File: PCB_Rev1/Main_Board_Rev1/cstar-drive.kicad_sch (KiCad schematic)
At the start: 2 parts, among them J12 532610771, J9 532610771

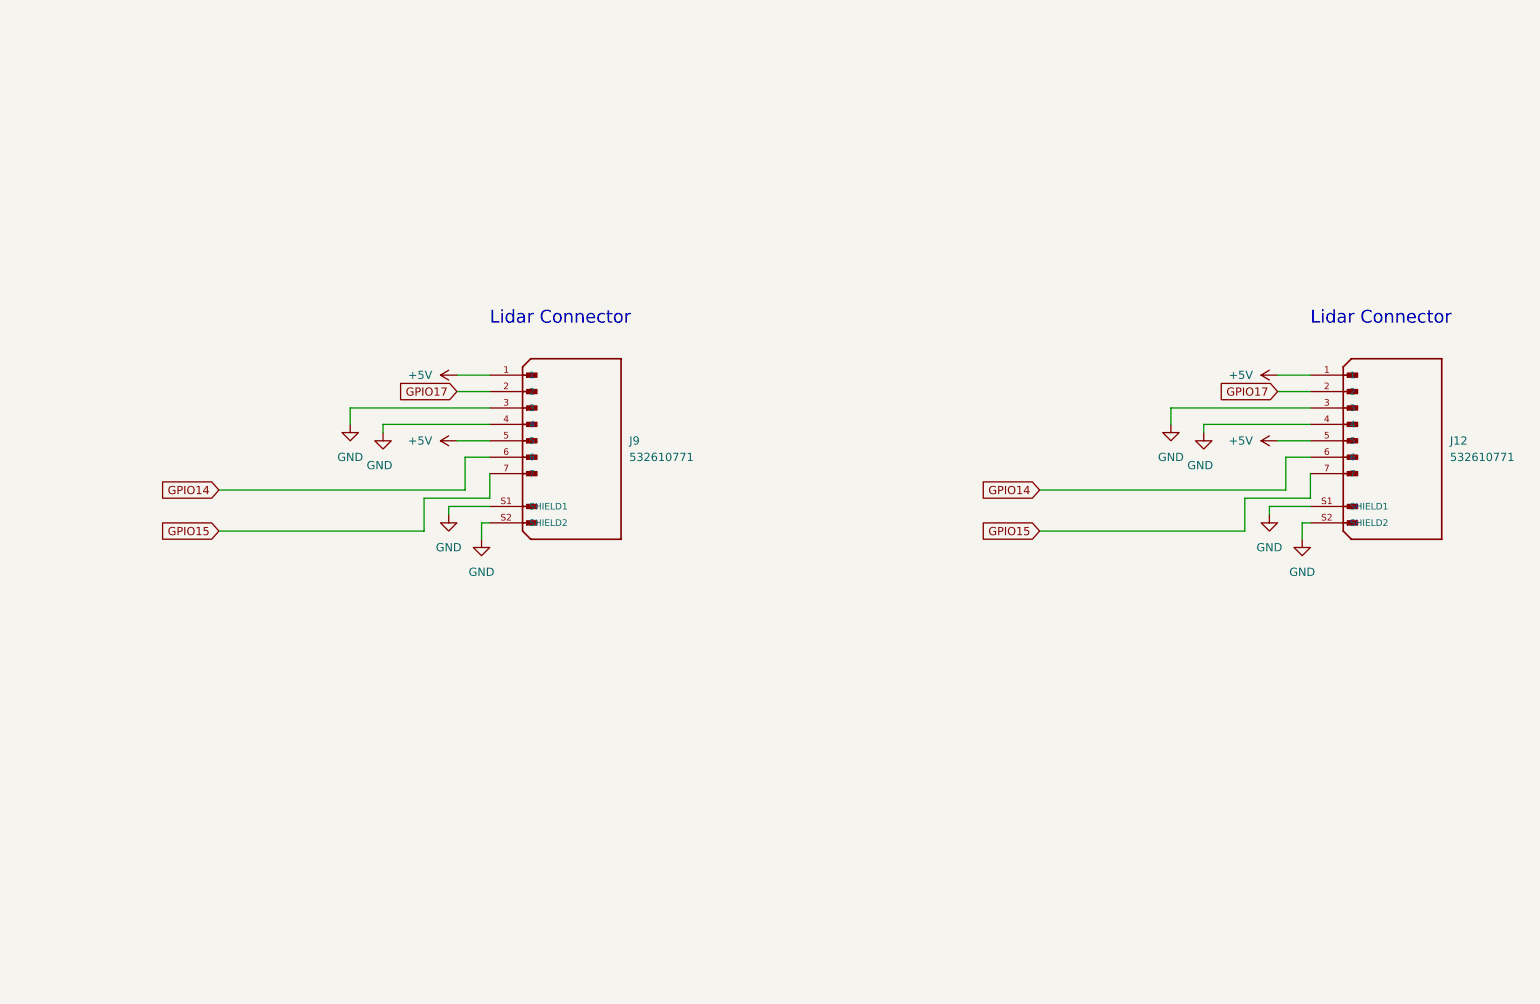
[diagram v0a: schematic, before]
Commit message: Revert "Audio subsystem re-created"
This reverts commit 6dc47edf88eae56b01440ce5f2dfd5da155ce597.
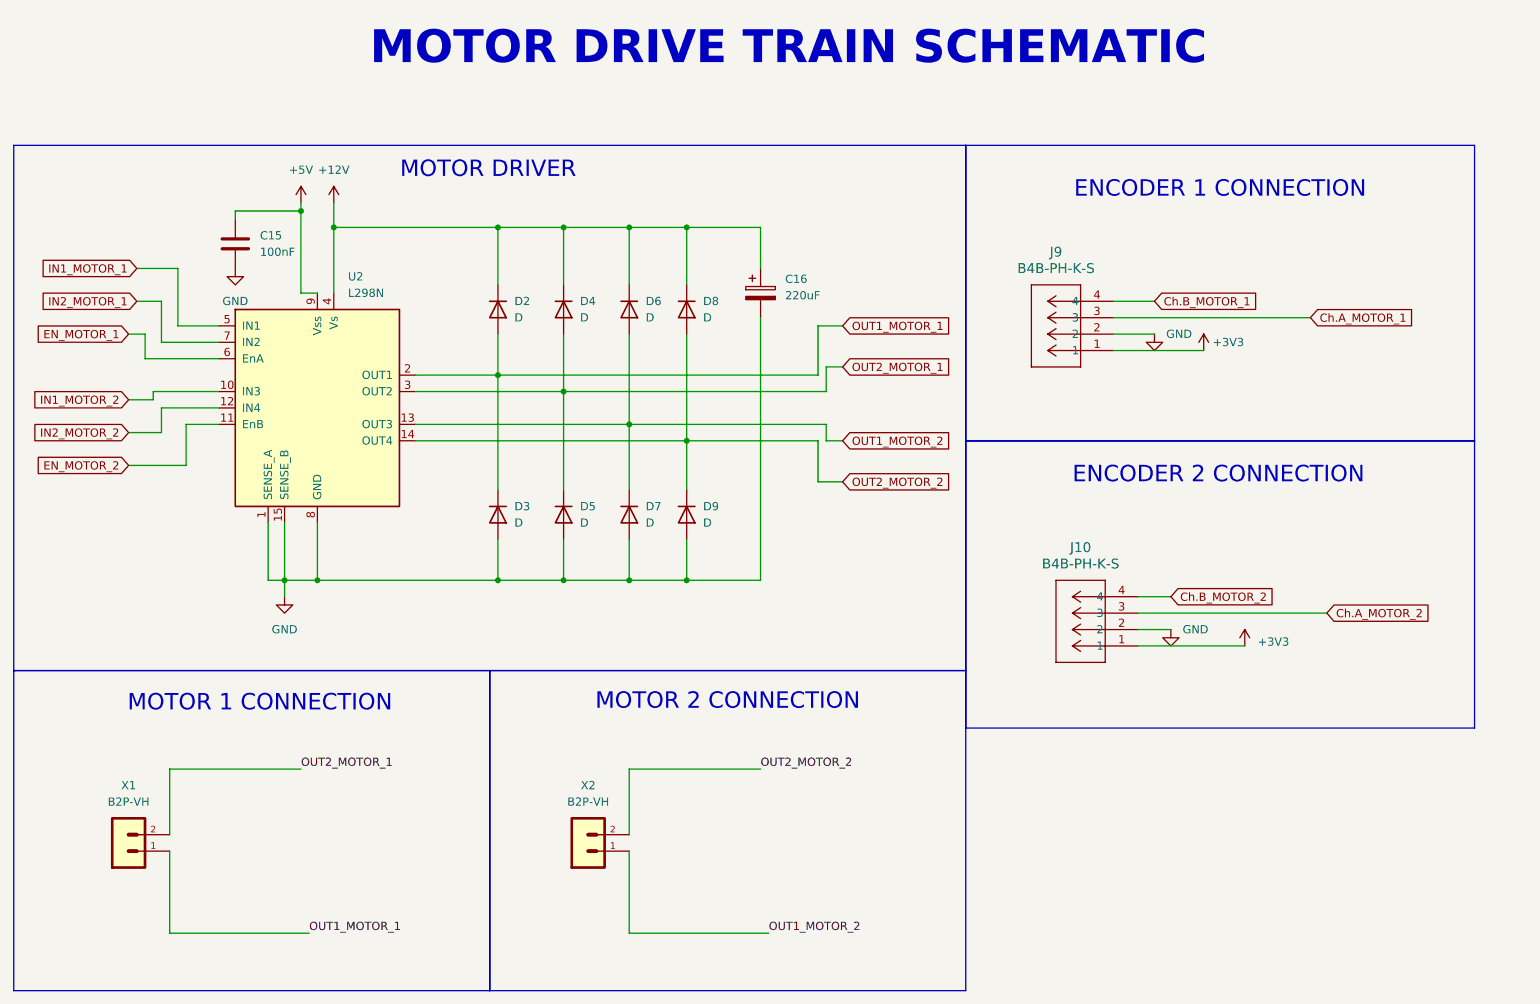
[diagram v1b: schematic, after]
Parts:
- removed J12, J9: 532610771, Connector_Molex:Molex_PicoBlade_53261-0771_1x07-1MP_P1.25mm_Horizontal, symbol 532610771:532610771
- added C15: 100nF, Capacitor_SMD:C_0805_2012Metric, symbol Device:C
- added C16: 220uF, Footprints:Cap_Polarized_220uF, symbol Device:C_Polarized
- added D2, D3, D4, D5, D6, D7, D8, D9: D, Footprints:Diode_1N4007, symbol Device:D
- added J10, J9: B4B-PH-K-S, Footprints:B4B_PH_K_S, symbol B4B_PH_K_S:B4B-PH-K-S
- added U2: L298N, Package_TO_SOT_THT:TO-220-15_P2.54x2.54mm_StaggerOdd_Lead4.58mm_Vertical, symbol Driver_Motor:L298N
- added X1, X2: B2P-VH, Footprints:B2P-VH, symbol B2P-VH:B2P-VH
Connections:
- net +5V: now also C15.1, U2.9 (Vss)
- net GND: now also C15.2, C16.2, D3.2 (A), D5.2 (A), D7.2 (A), D9.2 (A), J10.2, J9.2, U2.1 (SENSE_A), U2.15 (SENSE_B), U2.8 (GND)
- new net +12V: C16.1, D2.1 (K), D4.1 (K), D6.1 (K), D8.1 (K), U2.4 (Vs)
- new net +3V3: J10.1, J9.1
- new net Ch.A_MOTOR_1: J9.3
- new net Ch.A_MOTOR_2: J10.3
- new net Ch.B_MOTOR_1: J9.4
- new net Ch.B_MOTOR_2: J10.4
- new net EN_MOTOR_1: U2.6 (EnA)
- new net EN_MOTOR_2: U2.11 (EnB)
- new net IN1_MOTOR_1: U2.5 (IN1)
- new net IN1_MOTOR_2: U2.10 (IN3)
- new net IN2_MOTOR_1: U2.7 (IN2)
- new net IN2_MOTOR_2: U2.12 (IN4)
- new net OUT1_MOTOR_1: D2.2 (A), D3.1 (K), U2.2 (OUT1), X1.1
- new net OUT1_MOTOR_2: D6.2 (A), D7.1 (K), U2.13 (OUT3), X2.1
- new net OUT2_MOTOR_1: D4.2 (A), D5.1 (K), U2.3 (OUT2), X1.2
- new net OUT2_MOTOR_2: D8.2 (A), D9.1 (K), U2.14 (OUT4), X2.2
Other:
- note added: "ENCODER 1 CONNECTION"
- note added: "ENCODER 2 CONNECTION"
- note added: "MOTOR 1 CONNECTION"
- note added: "MOTOR 2 CONNECTION"
- note added: "MOTOR DRIVE TRAIN SCHEMATIC"
- note added: "MOTOR DRIVER"
- note removed: "Lidar Connector"
